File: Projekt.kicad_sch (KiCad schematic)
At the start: 98 parts, among them J1 Solar, J2 Battery, J3 USB_B_Mini, J4 INTERFACE PORT, J5 FAN, J6 JTAG, Q1 CSD19505KCS, Q1b1 CSD19505KCS, Q2 CSD19505KCS, Q2b1 CSD19505KCS, Q3 CSD19505KCS, Q3b1 CSD19505KCS, Q4 Si2306, Q5 MMBT3904 1A, Q6 MMBT3904 1A, Q7 Si2306, U1 ACS712, U10 ADS1015, U2 B1212S, U3 AMS1117-5.0, U4 AMS1117-3.3, U5 XL7005A, U6 XL7005A, U7 IR2104, U8 ESP32, U9 CH340G

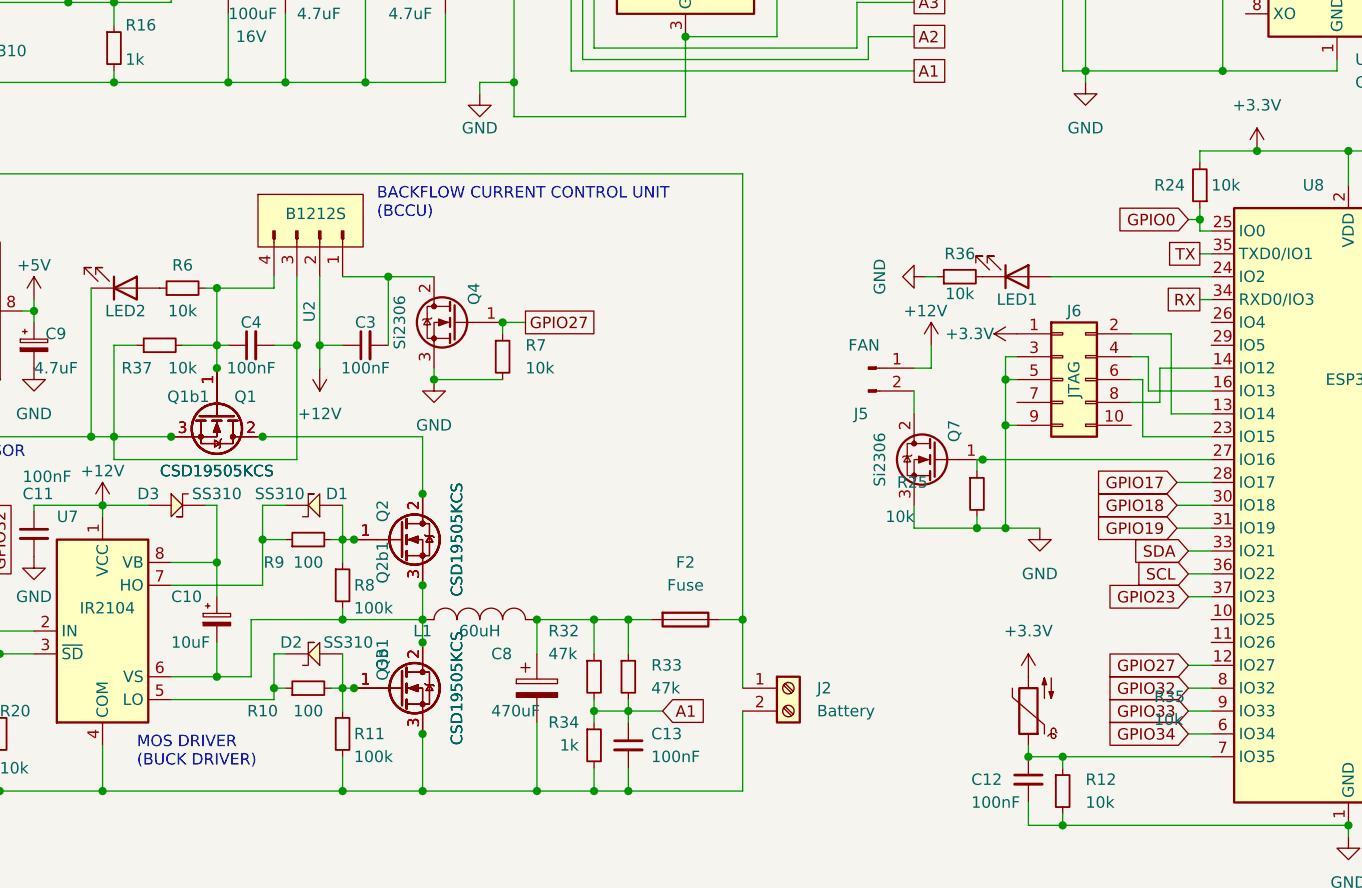
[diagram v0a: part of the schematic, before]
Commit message: Eigentlich okay...
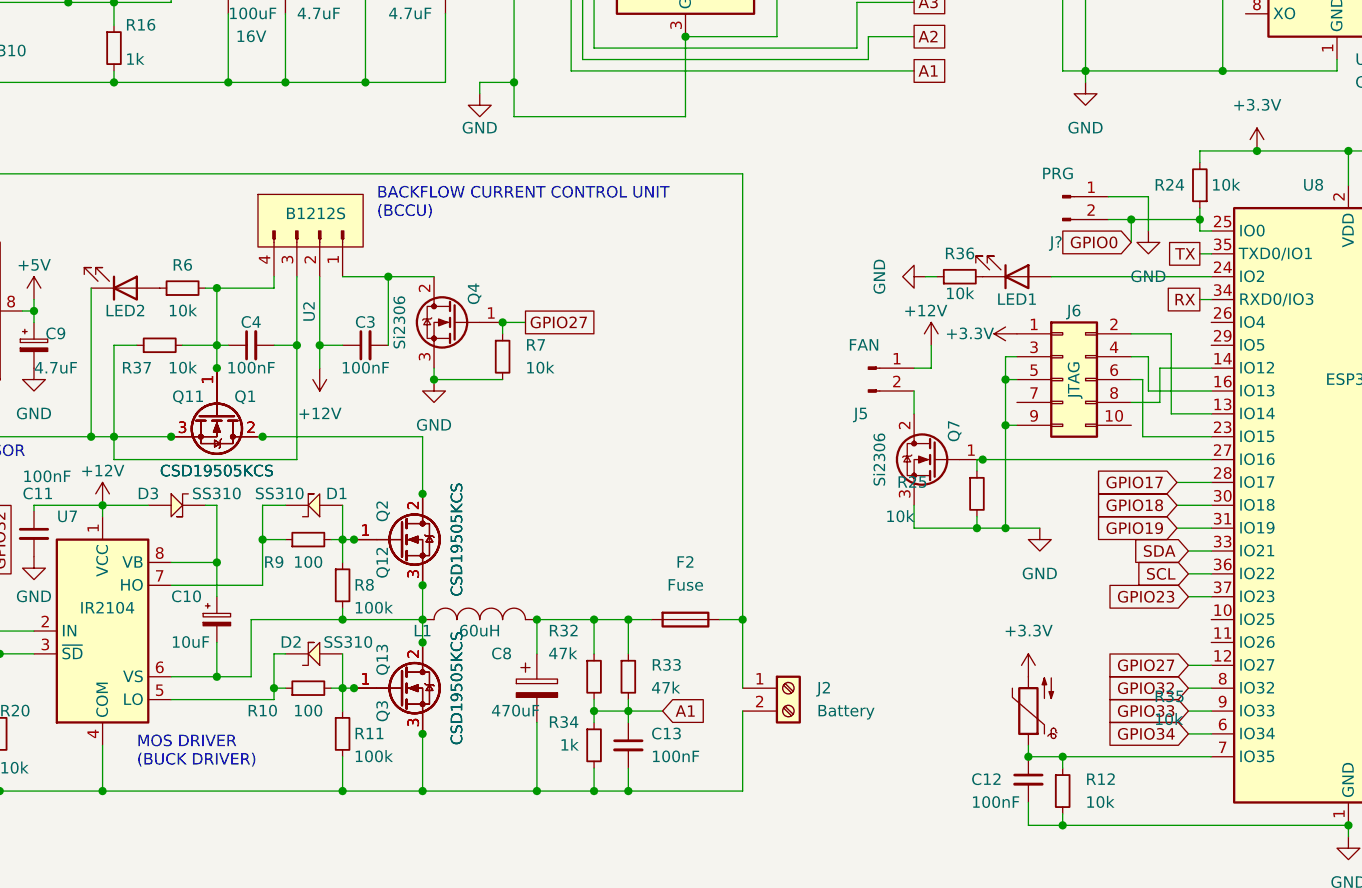
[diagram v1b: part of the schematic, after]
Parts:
- added J?: PRG, Connector_PinHeader_2.54mm:PinHeader_1x02_P2.54mm_Vertical, symbol Connector:Conn_01x02_Male
- renumbered Q1b1 to Q11, Q2b1 to Q12, Q3b1 to Q13
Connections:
- net GND: now also J?.1 (Pin_1)
- net GPIO0: now also J?.2 (Pin_2)
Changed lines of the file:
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@@
   (junction (at 44.45 154.94) (diameter 0) (color 0 0 0 0)
   )
+  (junction (at 185.42 91.44) (diameter 0) (color 0 0 0 0)
+  )
   (junction (at 86.36 24.13) (diameter 0) (color 0 0 0 0)
   )
@@
     (stroke (width 0) (type default) (color 0 0 0 0))
   )
+  (wire (pts (xy 182.88 91.44) (xy 185.42 91.44))
+    (stroke (width 0) (type default) (color 0 0 0 0))
+  )
   (wire (pts (xy 119.38 135.89) (xy 119.38 139.7))
     (stroke (width 0) (type default) (color 0 0 0 0))
@@
     (stroke (width 0) (type default) (color 0 0 0 0))
   )
+  (wire (pts (xy 187.325 88.9) (xy 187.325 92.71))
+    (stroke (width 0) (type default) (color 0 0 0 0))
+  )
   (wire (pts (xy 25.4 115.57) (xy 20.32 115.57))
     (stroke (width 0) (type default) (color 0 0 0 0))
@@
     (stroke (width 0) (type default) (color 0 0 0 0))
   )
+  (wire (pts (xy 182.88 88.9) (xy 187.325 88.9))
+    (stroke (width 0) (type default) (color 0 0 0 0))
+  )
   (wire (pts (xy 125.73 72.39) (xy 154.94 72.39))
     (stroke (width 0) (type default) (color 0 0 0 0))
@@
     (stroke (width 0) (type default) (color 0 0 0 0))
   )
+  (wire (pts (xy 185.42 91.44) (xy 185.42 93.98))
+    (stroke (width 0) (type default) (color 0 0 0 0))
+  )
   (wire (pts (xy 162.56 97.79) (xy 163.83 97.79))
     (stroke (width 0) (type default) (color 0 0 0 0))
@@
     (stroke (width 0) (type default) (color 0 0 0 0))
   )
-  (wire (pts (xy 191.77 91.44) (xy 193.04 91.44))
+  (wire (pts (xy 185.42 91.44) (xy 193.04 91.44))
     (stroke (width 0) (type default) (color 0 0 0 0))
   )
@@
     )
   )
-  (global_label "GPIO0" (shape input) (at 191.77 91.44 180) (fields_autoplaced)
+  (global_label "GPIO0" (shape input) (at 185.42 93.98 180) (fields_autoplaced)
     (effects (font (size 1.27 1.27)) (justify right))
-    (property "Intersheet References" "${INTERSHEET_REFS}" (id 0) (at 183.6721 91.3606 0)
+    (property "Intersheet References" "${INTERSHEET_REFS}" (id 0) (at 177.3221 93.9006 0)
       (effects (font (size 1.27 1.27)) (justify right) hide)
     )
@@
   (symbol (lib_id "footprint:CSD19505KCS") (at 83.82 113.03 270) (unit 1)
     (in_bom yes) (on_board yes)
-    (property "Reference" "Q1b1" (id 0) (at 80.645 111.125 90))
+    (property "Reference" "Q11" (id 0) (at 80.645 111.125 90))
     (property "Value" "CSD19505KCS" (id 1) (at 83.82 119.38 90))
     (property "Footprint" "Package_TO_SOT_THT:TO-220-3_Vertical" (id 2) (at 68.834 121.412 90)
@@
   (symbol (lib_id "footprint:CSD19505KCS") (at 104.14 127 0) (unit 1)
     (in_bom yes) (on_board yes)
-    (property "Reference" "Q2b1" (id 0) (at 102.235 129.54 90))
+    (property "Reference" "Q12" (id 0) (at 102.235 129.54 90))
     (property "Value" "CSD19505KCS" (id 1) (at 110.49 127 90))
     (property "Footprint" "Package_TO_SOT_THT:TO-220-3_Vertical" (id 2) (at 112.522 141.986 90)
@@
   (symbol (lib_id "footprint:CSD19505KCS") (at 104.14 143.51 0) (unit 1)
     (in_bom yes) (on_board yes)
-    (property "Reference" "Q3" (id 0) (at 102.235 140.335 90))
+    (property "Reference" "Q3" (id 0) (at 102.235 146.05 90))
     (property "Value" "CSD19505KCS" (id 1) (at 110.49 143.51 90))
     (property "Footprint" "Package_TO_SOT_THT:TO-220-3_Vertical" (id 2) (at 112.522 158.496 90)
@@
     (pin "2")
   )
+  (symbol (lib_id "power:GND") (at 187.325 92.71 0) (unit 1)
+    (in_bom yes) (on_board yes) (fields_autoplaced)
+    (property "Reference" "#PWR?" (id 0) (at 187.325 99.06 0)
+      (effects (font (size 1.27 1.27)) hide)
+    )
+    (property "Value" "GND" (id 1) (at 187.325 97.79 0))
+    (property "Footprint" "" (id 2) (at 187.325 92.71 0)
+      (effects (font (size 1.27 1.27)) hide)
+    )
+    (property "Datasheet" "" (id 3) (at 187.325 92.71 0)
+      (effects (font (size 1.27 1.27)) hide)
+    )
+    (pin "1")
+  )
   (symbol (lib_id "Device:R_Small") (at 166.37 97.79 90) (unit 1)
     (in_bom yes) (on_board yes)
@@
     (pin "1")
   )
+  (symbol (lib_id "Connector:Conn_01x02_Male") (at 177.8 88.9 0) (unit 1)
+    (in_bom yes) (on_board yes)
+    (property "Reference" "J?" (id 0) (at 177.8 93.98 0)
+      (effects (font (size 1.27 1.27)) (justify right))
+    )
+    (property "Value" "PRG" (id 1) (at 179.07 86.36 0)
+      (effects (font (size 1.27 1.27)) (justify right))
+    )
+    (property "Footprint" "Connector_PinHeader_2.54mm:PinHeader_1x02_P2.54mm_Vertical" (id 2) (at 177.8 88.9 0)
+      (effects (font (size 1.27 1.27)) hide)
+    )
+    (property "Datasheet" "~" (id 3) (at 177.8 88.9 0)
+      (effects (font (size 1.27 1.27)) hide)
+    )
+    (pin "1")
+    (pin "2")
+  )
   (symbol (lib_id "Device:C_Small") (at 129.54 149.86 0) (unit 1)
     (in_bom yes) (on_board yes)
@@
   (symbol (lib_id "footprint:CSD19505KCS") (at 104.14 143.51 0) (unit 1)
     (in_bom yes) (on_board yes)
-    (property "Reference" "Q3b1" (id 0) (at 102.235 140.335 90))
+    (property "Reference" "Q13" (id 0) (at 102.235 140.335 90))
     (property "Value" "CSD19505KCS" (id 1) (at 110.49 143.51 90))
     (property "Footprint" "Package_TO_SOT_THT:TO-220-3_Vertical" (id 2) (at 112.522 158.496 90)
@@
       (reference "#PWR0125") (unit 1) (value "GND") (footprint "")
     )
+    (path "/c5a5ef8d-c592-47eb-bd21-ceec507b7d31"
+      (reference "#PWR?") (unit 1) (value "GND") (footprint "")
+    )
     (path "/6c036c9e-e0d1-4bac-b51b-db7b92cdf233"
       (reference "C1") (unit 1) (value "100nF") (footprint "Capacitor_SMD:C_0603_1608Metric")
@@
       (reference "J6") (unit 1) (value "JTAG") (footprint "Connector_PinHeader_1.27mm:PinHeader_2x05_P1.27mm_Vertical_SMD")
     )
+    (path "/d0f189fe-2700-4f77-8370-882eccb1f8d9"
+      (reference "J?") (unit 1) (value "PRG") (footprint "Connector_PinHeader_2.54mm:PinHeader_1x02_P2.54mm_Vertical")
+    )
     (path "/a34be4f0-cd07-4bab-9f46-bdfef665e51a"
       (reference "L1") (unit 1) (value "60uH") (footprint "Inductor_THT:L_Toroid_Vertical_L21.6mm_W11.4mm_P7.62mm_Pulse_KM-3")
@@
       (reference "Q1") (unit 1) (value "CSD19505KCS") (footprint "Package_TO_SOT_THT:TO-220-3_Vertical")
     )
-    (path "/068a26f9-efe8-4653-9ca9-597ae39bb735"
-      (reference "Q1b1") (unit 1) (value "CSD19505KCS") (footprint "Package_TO_SOT_THT:TO-220-3_Vertical")
-    )
     (path "/539c37cf-e417-4bd0-89c6-457ec992b15f"
       (reference "Q2") (unit 1) (value "CSD19505KCS") (footprint "Package_TO_SOT_THT:TO-220-3_Vertical")
     )
-    (path "/54409513-d3fa-492e-a001-a088fdce9fa5"
-      (reference "Q2b1") (unit 1) (value "CSD19505KCS") (footprint "Package_TO_SOT_THT:TO-220-3_Vertical")
-    )
     (path "/bb113282-5d8f-4b0b-a4b8-2446b034aad5"
       (reference "Q3") (unit 1) (value "CSD19505KCS") (footprint "Package_TO_SOT_THT:TO-220-3_Vertical")
     )
-    (path "/dd65f54c-87a0-4385-98b4-810c8b6410c7"
-      (reference "Q3b1") (unit 1) (value "CSD19505KCS") (footprint "Package_TO_SOT_THT:TO-220-3_Vertical")
-    )
     (path "/d518002e-8259-4f21-880a-acde968c86e4"
       (reference "Q4") (unit 1) (value "Si2306") (footprint "Package_TO_SOT_SMD:SOT-23")
@@
       (reference "Q7") (unit 1) (value "Si2306") (footprint "Package_TO_SOT_SMD:SOT-23")
     )
+    (path "/068a26f9-efe8-4653-9ca9-597ae39bb735"
+      (reference "Q11") (unit 1) (value "CSD19505KCS") (footprint "Package_TO_SOT_THT:TO-220-3_Vertical")
+    )
+    (path "/54409513-d3fa-492e-a001-a088fdce9fa5"
+      (reference "Q12") (unit 1) (value "CSD19505KCS") (footprint "Package_TO_SOT_THT:TO-220-3_Vertical")
+    )
+    (path "/dd65f54c-87a0-4385-98b4-810c8b6410c7"
+      (reference "Q13") (unit 1) (value "CSD19505KCS") (footprint "Package_TO_SOT_THT:TO-220-3_Vertical")
+    )
     (path "/c953cab7-4946-4acc-9567-3e799c6ea44c"
